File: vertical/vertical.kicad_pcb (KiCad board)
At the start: 2 copper layers, 26 x 27 mm, 15 parts, among them J1 internal, J2 PROG, U1 LM1117-3.3, U2 ESP32-C3-WROOM-02, U5 MAX485E

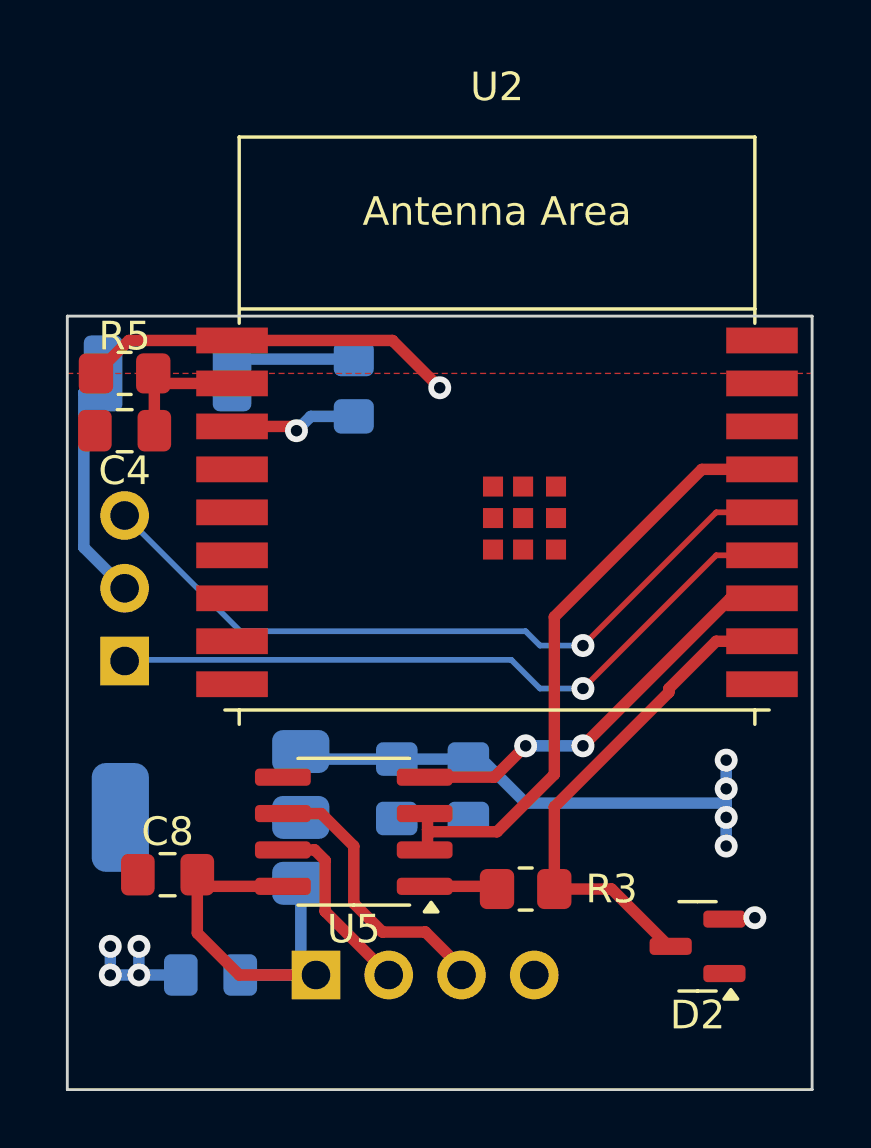
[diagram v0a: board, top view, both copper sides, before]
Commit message: Update KiCad design files
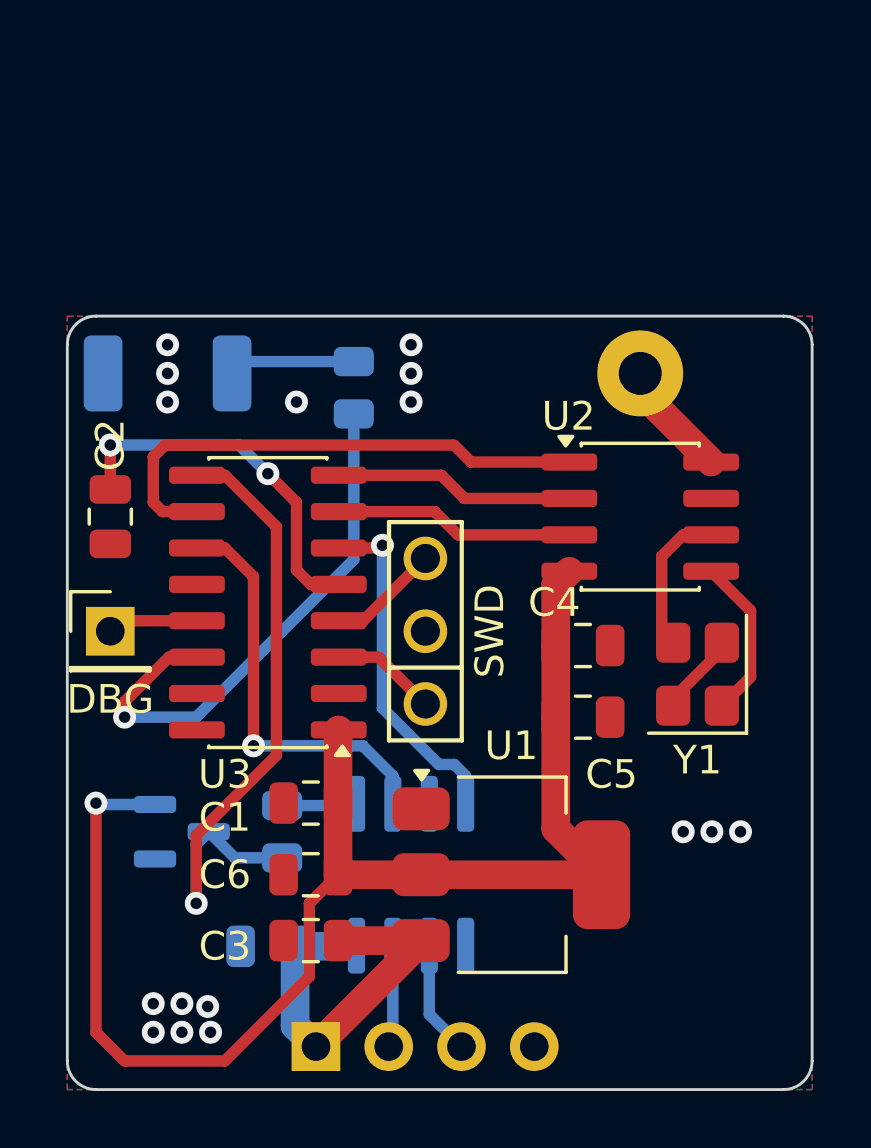
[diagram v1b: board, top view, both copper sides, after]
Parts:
- removed the J2 at (127.0, 77.0)
- removed R5: 10k, Resistor_SMD:R_0805_2012Metric_Pad1.20x1.40mm_HandSolder
- added A1: 31mm, Drake:Wire antena 2.4GHz, F.Cu at (145.0, 67.0)
- added C5: 100n, Capacitor_SMD:C_0805_2012Metric, F.Cu at (143.0, 79.0)
- added C6: 10u, Capacitor_SMD:C_0805_2012Metric, F.Cu at (133.5, 84.5)
- added J1: DBG, Connector_PinHeader_2.54mm:PinHeader_1x01_P2.54mm_Vertical, F.Cu at (126.5, 76.0)
- added U3: PY32F003W1xSx, Package_SO:SOIC-16_3.9x9.9mm_P1.27mm, F.Cu at (132.0, 75.0)
- added X1: SWD, Drake:SWD, F.Cu at (137.5, 76.0)
- added Y1: 16MHz, Crystal:Crystal_SMD_3225-4Pin_3.2x2.5mm, F.Cu at (147.0, 77.5)
- C1: value 10u -> 100n; footprint Capacitor_SMD:C_0805_2012Metric_Pad1.18x1.45mm_HandSolder -> Capacitor_SMD:C_0805_2012Metric; moved to F.Cu
- C2: value 47u -> 100n; footprint Capacitor_SMD:C_0805_2012Metric_Pad1.18x1.45mm_HandSolder -> Capacitor_SMD:C_0805_2012Metric; moved to F.Cu
- C3: value 47u -> 10u; footprint Capacitor_SMD:C_0805_2012Metric_Pad1.18x1.45mm_HandSolder -> Capacitor_SMD:C_0805_2012Metric; moved to F.Cu
- C4: footprint Capacitor_SMD:C_0805_2012Metric_Pad1.18x1.45mm_HandSolder -> Capacitor_SMD:C_0805_2012Metric
- C7: renamed from C8; footprint Capacitor_SMD:C_0805_2012Metric_Pad1.18x1.45mm_HandSolder -> Capacitor_SMD:C_0805_2012Metric; moved to B.Cu
- D1: renamed from D2; moved to B.Cu
- R1: renamed from R3; footprint Resistor_SMD:R_0805_2012Metric_Pad1.20x1.40mm_HandSolder -> Resistor_SMD:R_0805_2012Metric; moved to B.Cu
- R2: renamed from R1; value 270R -> 330R; footprint Resistor_SMD:R_0805_2012Metric_Pad1.20x1.40mm_HandSolder -> Resistor_SMD:R_0805_2012Metric
- U1: value LM1117-3.3 -> LM1117MP-3.3; moved to F.Cu
- U2: value ESP32-C3-WROOM-02 -> PAN2110P0AA; footprint Drake:ESP32-C3-WROOM-02-Handsolder -> Package_SO:SOIC-8_3.9x4.9mm_P1.27mm
- U4: renamed from U5; moved to B.Cu
- moved D1 18.4 mm to (129.0, 83.0), turned to 0 degrees
- moved C4 17.7 mm to (143.0, 76.5), turned to 0 degrees
- moved C2 13.8 mm to (126.5, 72.0), turned to -90 degrees
- moved U1 10.7 mm to (140.5, 84.5), turned to 0 degrees
- moved R1 8.73 mm to (132.5, 83.0), turned to 90 degrees
- moved C3 7.64 mm to (133.5, 86.8), turned to 180 degrees
- moved C1 6.95 mm to (133.5, 82.0)
- moved U2 5.39 mm to (145.0, 72.0)
- moved C7 4.30 mm to (132.0, 87.0)
- moved J2 2.50 mm to (133.7, 90.5)
- moved U4 2.50 mm to (137.0, 84.5), turned to -90 degrees
- renumbered D1 to D2, J1 to J2
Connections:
- net /RX renamed Net-(U4-RO)
- C1 pad 1: +5V -> +3V3
- C2 pad 1: +3V3 -> Net-(U3-PF0/PF2-NRST)
- C3 pad 1: +3V3 -> +5V
- C4 pad 1: Net-(U2-EN/CHIP_PU) -> +3V3
- D1 pad 3: Net-(D2-COM) -> /RS485_RX
- R1 pad 1: Net-(D2-COM) -> /RS485_RX
- U2 pad 1: +3V3 -> /~{RF_CS}
- U2 pad 2: Net-(U2-EN/CHIP_PU) -> /RF_SCK
- U2 pad 3: /LED -> /RF_DATA
- U2 pad 4: unconnected-(U2-GPIO5/ADC2_CH0-Pad4) -> +3V3
- U2 pad 5: unconnected-(U2-GPIO6-Pad5) -> Net-(U2-XC1)
- U2 pad 6: unconnected-(U2-GPIO7-Pad6) -> Net-(U2-XC0)
- U2 pad 7: unconnected-(U2-GPIO8-Pad7) -> GND
- U2 pad 8: unconnected-(U2-GPIO9-Pad8) -> Net-(A1-A)
- U4 pad 2: /TXEN -> /RS485_TXEN
- U4 pad 3: /TXEN -> /RS485_TXEN
- U4 pad 4: /TX -> /RS485_TX
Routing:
- net +3V3: track 13.7 -> 48.9 mm, vias 2 -> 1
- net GND: track 31.4 -> 2.90 mm, vias 8 -> 16
- net /USB_D+: track 25.6 -> 0.00 mm, vias 1 -> 0
- net /USB_D-: track 24.1 -> 0.00 mm, vias 1 -> 0
- net /RS485_RX: track 0.00 -> 23.4 mm, vias 0 -> 1
- net /TXEN: track 20.9 -> 0.00 mm
- net /~{RF_CS}: track 0.00 -> 18.1 mm
- net Net-(D2-COM): track 17.0 -> 0.00 mm
- net /RS485_TXEN: track 0.00 -> 15.8 mm, vias 0 -> 1
- net /LED: track 4.02 -> 19.1 mm
- net /TX: track 13.9 -> 0.00 mm, vias 2 -> 0
- net Net-(U3-PF0/PF2-NRST): track 0.00 -> 12.9 mm, vias 0 -> 2
- net /RS485_TX: track 0.00 -> 12.1 mm, vias 0 -> 1
- net /RF_DATA: track 0.00 -> 8.39 mm
- net /RF_SCK: track 0.00 -> 8.39 mm
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- added copper zone on B.Cu, net GND
- removed copper zone on B.Cu, net +3V3
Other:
- outline, holes or cut-outs redrawn
- board text added: "RS485 WiFi v2.2 drake.cz"
- board text removed: "EDA&TATA"
- board text removed: "RS485 WiFi v1.2"
